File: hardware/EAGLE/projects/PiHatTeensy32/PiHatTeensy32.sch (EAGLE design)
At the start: 15 parts, among them T4 BM08B-SRSS-TB, U1 TSR_1-2450, X1 RASPI_BOARD_B+_H

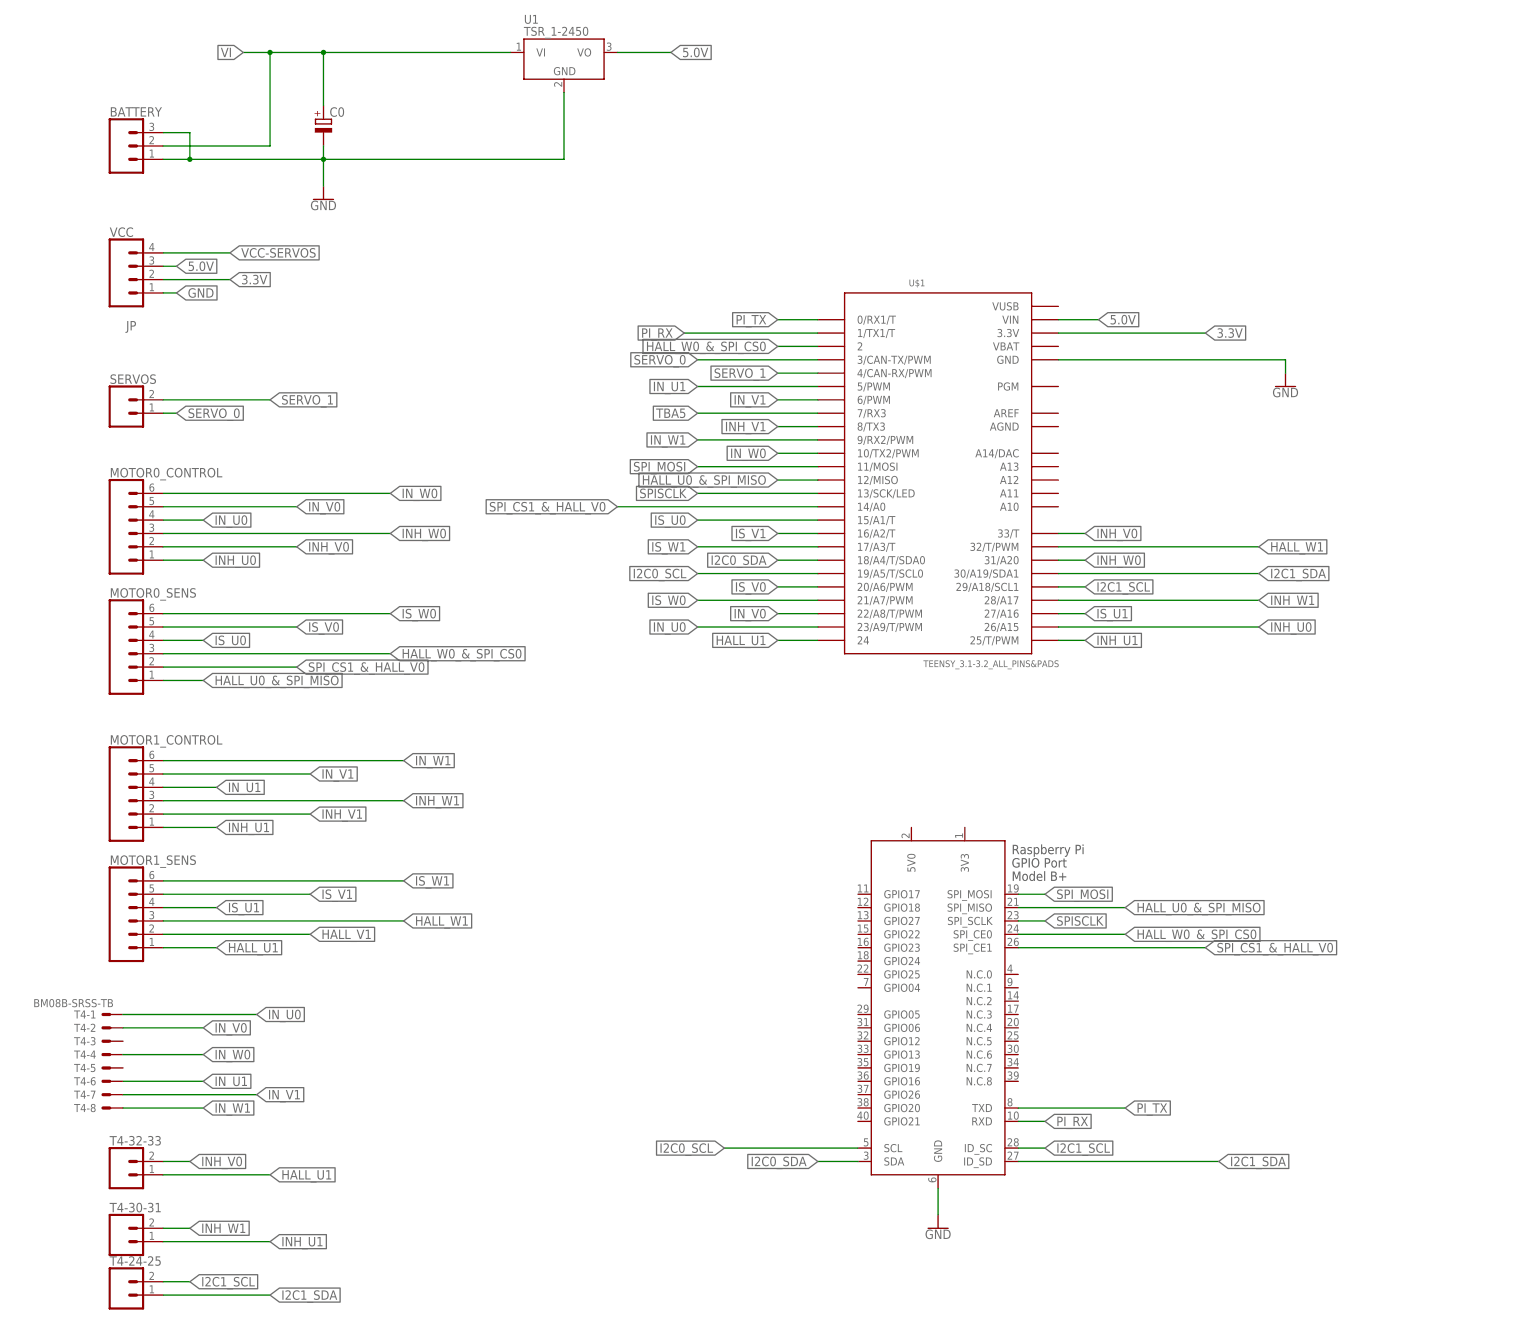
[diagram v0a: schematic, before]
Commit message: Befour autorouting
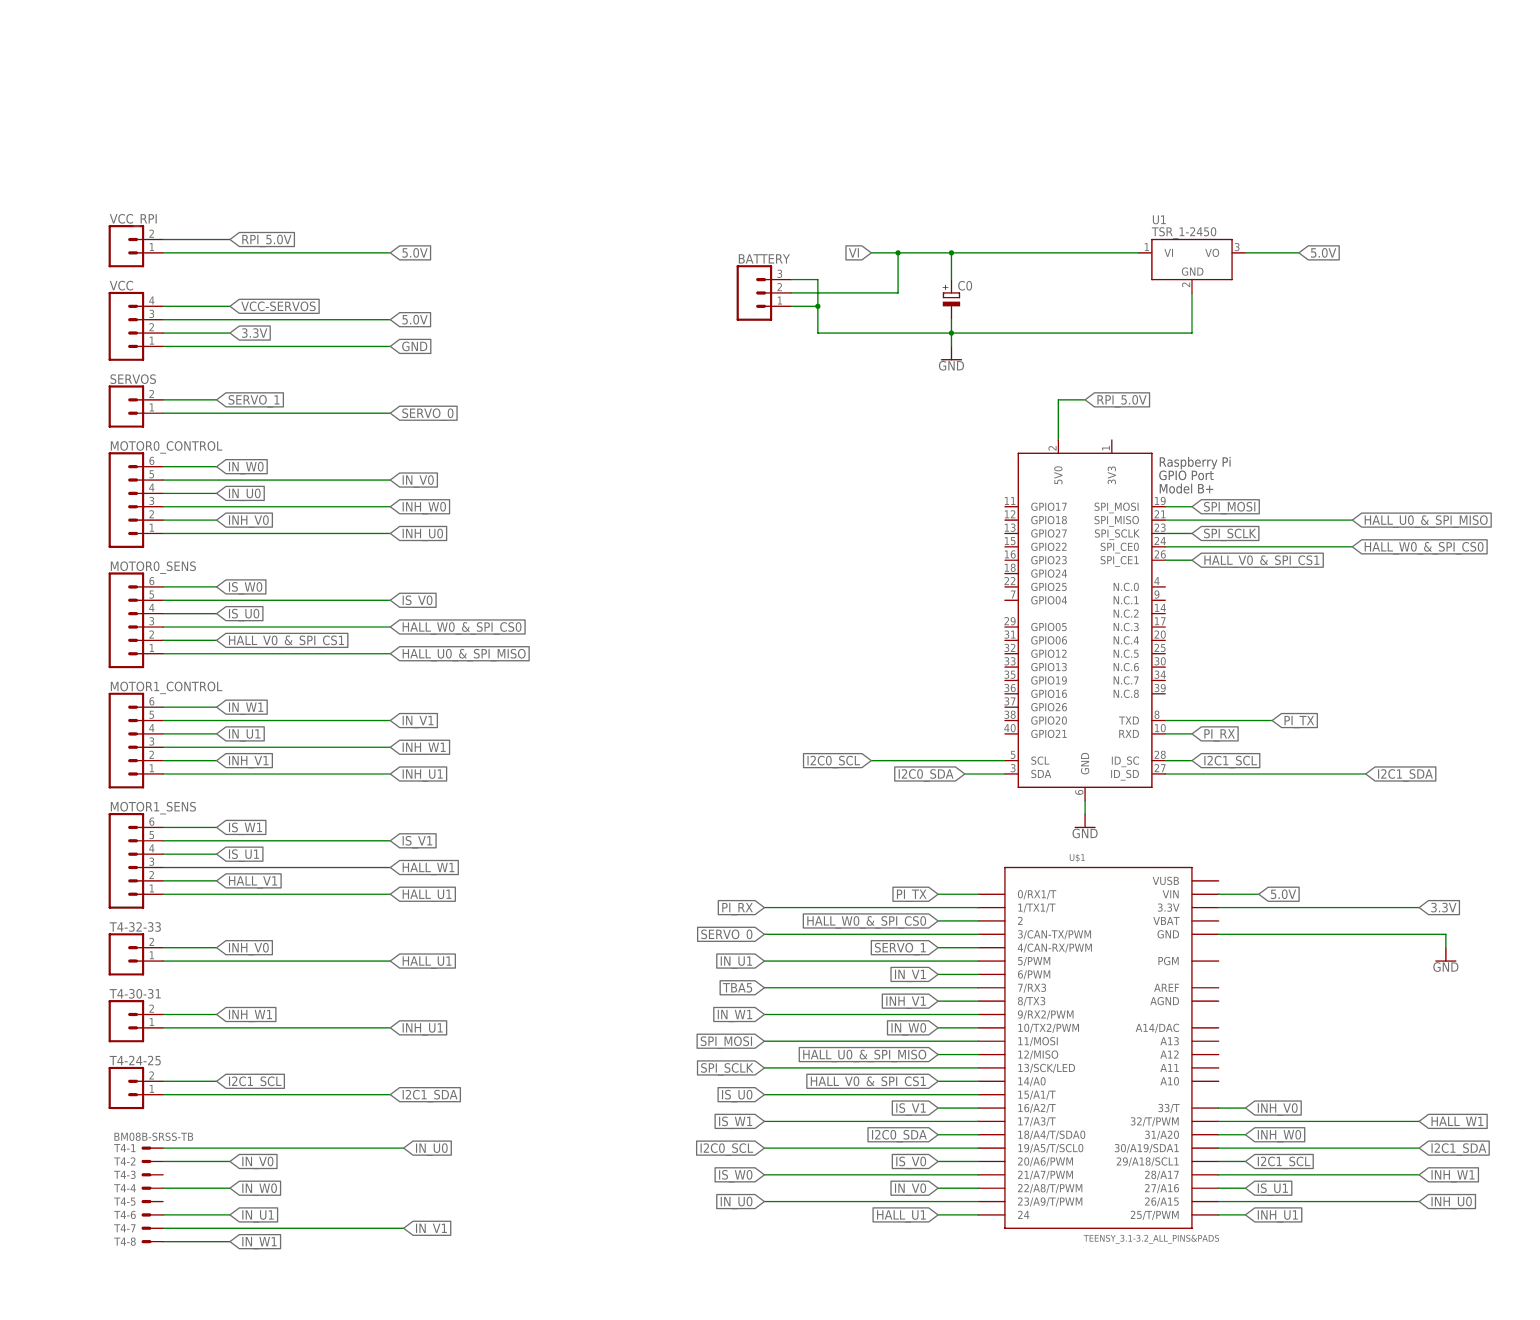
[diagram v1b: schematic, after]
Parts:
- added VCC_RPI: (no value), SparkFun-Connectors:CONN_021X02_NO_SILK
- VCC: value JP -> (none)
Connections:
- net SPISCLK renamed SPI_SCLK
- net SPI_CS1_&_HALL_V0 renamed HALL_V0_&_SPI_CS1
- new net RPI_5.0V: VCC_RPI.2, X1.5V0
- net 5.0V: now also VCC_RPI.1
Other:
- moved on the sheet: BATTERY, C0, MOTOR0_CONTROL, MOTOR0_SENS, MOTOR1_CONTROL, MOTOR1_SENS, T4-1, T4-2, T4-24-25, T4-3, T4-30-31, T4-32-33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
